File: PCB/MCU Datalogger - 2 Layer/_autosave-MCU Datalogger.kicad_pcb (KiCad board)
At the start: 2 copper layers, 50.7 x 30.4 mm, 29 parts, among them J1 Conn_01x04_Pin, J2 Conn_01x04_Pin, J3 Conn_01x09_Pin, J4 Conn_02x03_Odd_Even, U1 24LC1025, U2 24LC1025, U3 DS1337S+, U4 ATMEGA328P-AU, Y1 16 MHz, Y2 32.768 Khz

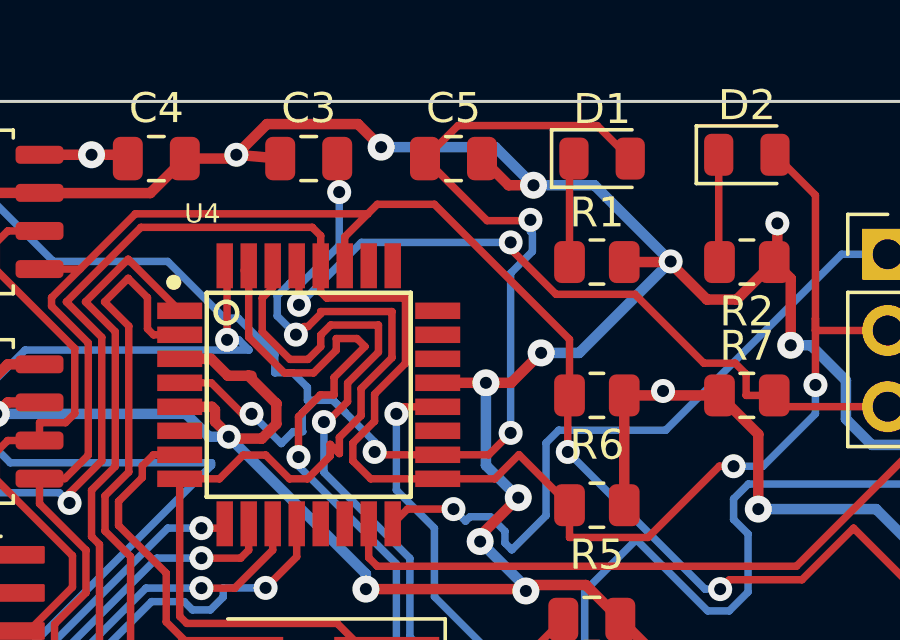
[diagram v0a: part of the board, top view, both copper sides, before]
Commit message: routing
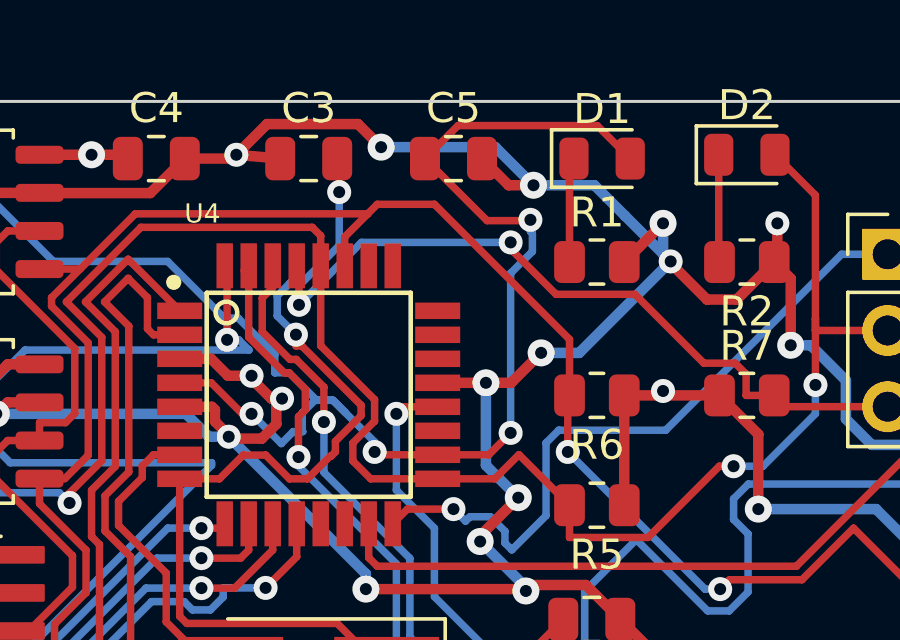
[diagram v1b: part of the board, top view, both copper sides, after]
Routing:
- net /TX: track 37.4 -> 32.3 mm
- net /RX: track 81.5 -> 76.4 mm
- net Net-(U4-PB7): track 35.6 -> 31.3 mm
- net /SCK: track 104.9 -> 102.5 mm
- net GND: track 168.8 -> 170.8 mm, vias 20 -> 23
